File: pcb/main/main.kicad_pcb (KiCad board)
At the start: 2 copper layers, 29.4 x 98.3 mm, 54 parts, among them J1 Conn_01x04, J2 USB_B, J3 Serial, J4 STLink, J5 RJ45, J6 SELECT, J7 READ, J8 TRACKBALL, SW5 RST_SW, SW6 BOOT0, SW7 BOOT1, U1 3.3v regul, U2 STM32F103C8Tx, Y1 32.768kHz, Y2 8MHz

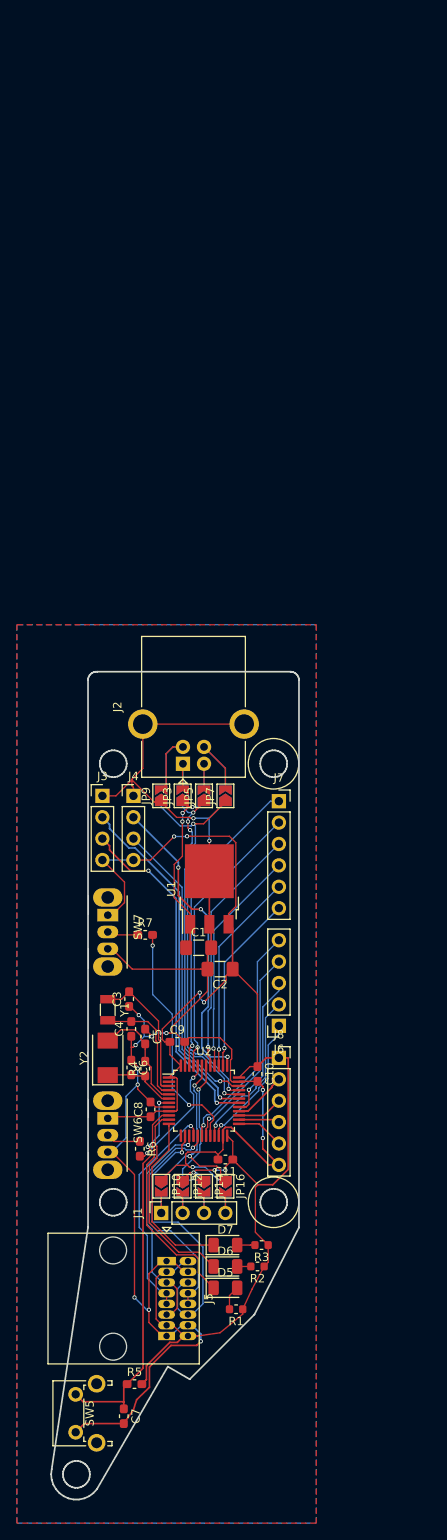
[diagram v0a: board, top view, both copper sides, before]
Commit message: fix pcb
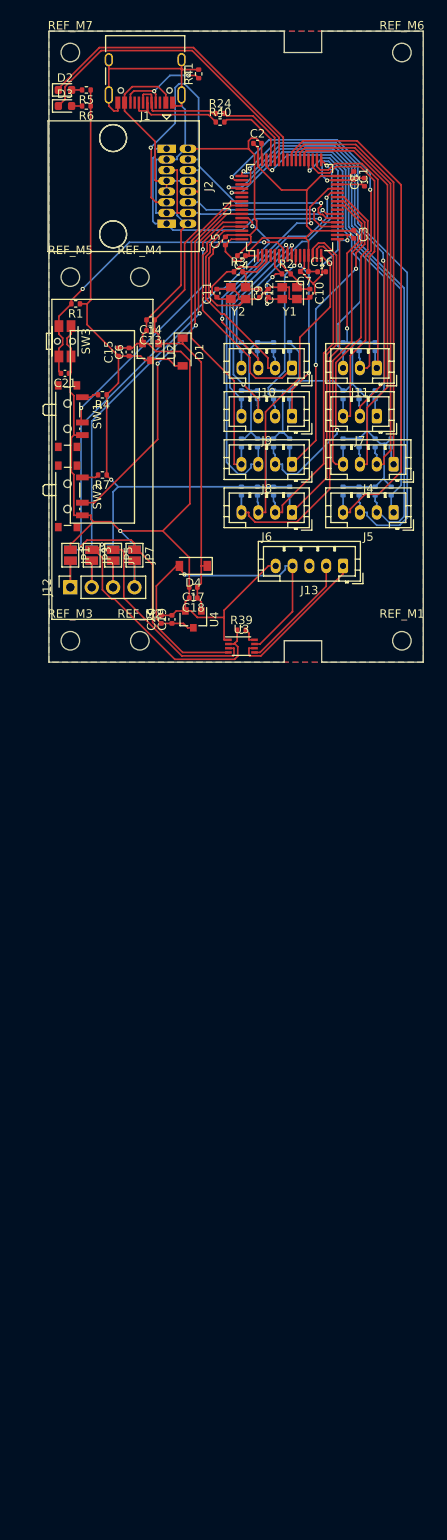
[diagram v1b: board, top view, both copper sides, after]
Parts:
- removed D5, D6, D7: LED, LED_SMD:LED_1206_3216Metric
- removed G*** (x2): LOGO, folivora:logo
- removed JP10, JP12, JP14, JP16, JP9: R, Jumper:SolderJumper-2_P1.3mm_Open_TrianglePad1.0x1.5mm
- removed JP11, JP13, JP15, JP17: L, Jumper:SolderJumper-2_P1.3mm_Open_TrianglePad1.0x1.5mm
- removed SW5: RST_SW, Button_Switch_THT:SW_Tactile_SPST_Angled_PTS645Vx31-2LFS
- removed SW6: BOOT0, Button_Switch_THT:SW_CuK_OS102011MA1QN1_SPDT_Angled
- removed SW7: BOOT1, Button_Switch_THT:SW_CuK_OS102011MA1QN1_SPDT_Angled
- added C12: C, Capacitor_SMD:C_0402_1005Metric, F.Cu at (25.0, -43.8)
- added C13: 1uF, Capacitor_SMD:C_0402_1005Metric, F.Cu at (12.1, -39.4)
- added C14: 0.1uF, Capacitor_SMD:C_0402_1005Metric, F.Cu at (12.1, -40.6)
- added C15: 0.1uF, Capacitor_SMD:C_0402_1005Metric, F.Cu at (8.26, -36.8)
- added C16: 1uF, Capacitor_SMD:C_0402_1005Metric, F.Cu at (32.4, -46.4)
- added C17: 1uF, Capacitor_SMD:C_0402_1005Metric, F.Cu at (17.1, -8.89)
- added C18: 0.1uF, Capacitor_SMD:C_0402_1005Metric, F.Cu at (17.1, -7.62)
- added C19: 0.1uF, Capacitor_SMD:C_0402_1005Metric, F.Cu at (14.6, -5.08)
- added C20: 1uF, Capacitor_SMD:C_0402_1005Metric, F.Cu at (13.3, -5.08)
- added C21: 0.1uF, Capacitor_SMD:C_0402_1005Metric, F.Cu at (1.91, -34.3)
- added D1: SBD, Diode_SMD:D_SOD-123, F.Cu at (15.9, -36.8)
- added D2: Error, LED_SMD:LED_0603_1608Metric, F.Cu at (1.91, -67.9)
- added D3: Status, LED_SMD:LED_0603_1608Metric, F.Cu at (1.91, -66.0)
- added D4: SBD, Diode_SMD:D_SOD-123, F.Cu at (17.1, -11.4)
- added J10: COL4, Connector_JST:JST_PH_B4B-PH-K_1x04_P2.00mm_Vertical, F.Cu at (28.9, -34.9)
- added J11: COL6, Connector_JST:JST_PH_B3B-PH-K_1x03_P2.00mm_Vertical, F.Cu at (38.9, -34.9)
- added J12: OLED, folivora:OLED, F.Cu at (6.35, -8.89)
- added J13: Conn_01x05_Female, Connector_JST:JST_PH_B5B-PH-K_1x05_P2.00mm_Vertical, F.Cu at (34.9, -11.4)
- added J9: COL3, Connector_JST:JST_PH_B4B-PH-K_1x04_P2.00mm_Vertical, F.Cu at (28.9, -29.2)
- added JP1: OLED_1_F, Jumper:SolderJumper-2_P1.3mm_Open_Pad1.0x1.5mm, F.Cu at (2.54, -12.7)
- added R10: 10k, Resistor_SMD:R_0402_1005Metric, B.Cu at (36.8, -20.3)
- added R11: 10k, Resistor_SMD:R_0402_1005Metric, B.Cu at (34.9, -20.3)
- added R12: 10k, Resistor_SMD:R_0402_1005Metric, B.Cu at (40.6, -26.0)
- added R13: 10k, Resistor_SMD:R_0402_1005Metric, B.Cu at (38.7, -26.0)
- added R14: 10k, Resistor_SMD:R_0402_1005Metric, B.Cu at (36.8, -26.0)
- added R15: 10k, Resistor_SMD:R_0402_1005Metric, B.Cu at (34.9, -26.0)
- added R16: 10k, Resistor_SMD:R_0402_1005Metric, B.Cu at (28.6, -31.8)
- added R17: 10k, Resistor_SMD:R_0402_1005Metric, B.Cu at (26.7, -31.8)
- added R18: 10k, Resistor_SMD:R_0402_1005Metric, B.Cu at (24.8, -31.8)
- added R19: 10k, Resistor_SMD:R_0402_1005Metric, B.Cu at (22.9, -31.8)
- added R20: 10k, Resistor_SMD:R_0402_1005Metric, B.Cu at (34.9, -37.5)
- added R21: 10k, Resistor_SMD:R_0402_1005Metric, B.Cu at (36.8, -37.5)
- added R22: 10k, Resistor_SMD:R_0402_1005Metric, B.Cu at (38.7, -37.5)
- added R23: 10k, Resistor_SMD:R_0402_1005Metric, B.Cu at (22.9, -37.5)
- added R24: 10, Resistor_SMD:R_0402_1005Metric, F.Cu at (20.3, -65.2)
- added R25: 10k, Resistor_SMD:R_0402_1005Metric, B.Cu at (24.8, -37.5)
- added R26: 10k, Resistor_SMD:R_0402_1005Metric, B.Cu at (26.7, -37.5)
- added R27: 10k, Resistor_SMD:R_0402_1005Metric, B.Cu at (28.6, -37.5)
- added R28: 10k, Resistor_SMD:R_0402_1005Metric, B.Cu at (22.9, -26.0)
- added R29: 10k, Resistor_SMD:R_0402_1005Metric, B.Cu at (24.8, -26.0)
- added R30: 10k, Resistor_SMD:R_0402_1005Metric, B.Cu at (26.7, -26.0)
- added R31: 10k, Resistor_SMD:R_0402_1005Metric, B.Cu at (28.6, -26.0)
- added R32: 10k, Resistor_SMD:R_0402_1005Metric, B.Cu at (34.9, -31.8)
- added R33: 10k, Resistor_SMD:R_0402_1005Metric, B.Cu at (36.8, -31.8)
- added R34: 10k, Resistor_SMD:R_0402_1005Metric, B.Cu at (38.7, -31.8)
- added R35: 10k, Resistor_SMD:R_0402_1005Metric, B.Cu at (22.9, -20.3)
- added R36: 10k, Resistor_SMD:R_0402_1005Metric, B.Cu at (24.8, -20.3)
- added R37: 10k, Resistor_SMD:R_0402_1005Metric, B.Cu at (26.7, -20.3)
- added R38: 10k, Resistor_SMD:R_0402_1005Metric, B.Cu at (28.6, -20.3)
- added R39: R, Resistor_SMD:R_0402_1005Metric, F.Cu at (22.9, -3.81)
- added R40: 10, Resistor_SMD:R_0402_1005Metric, F.Cu at (20.3, -64.1)
- added R41: 5.1k, Resistor_SMD:R_0402_1005Metric, F.Cu at (17.8, -69.8)
- added R8: 10k, Resistor_SMD:R_0402_1005Metric, B.Cu at (40.6, -20.3)
- added R9: 10k, Resistor_SMD:R_0402_1005Metric, B.Cu at (38.7, -20.3)
- added REF_M1: MountingHole_2.2mm_M2, MountingHole:MountingHole_2.2mm_M2, F.Cu at (41.9, -2.54)
- added REF_M2: MountingHole_2.2mm_M2, MountingHole:MountingHole_2.2mm_M2, F.Cu at (10.8, -2.54)
- added REF_M3: MountingHole_2.2mm_M2, MountingHole:MountingHole_2.2mm_M2, F.Cu at (2.54, -2.54)
- added REF_M4: MountingHole_2.2mm_M2, MountingHole:MountingHole_2.2mm_M2, F.Cu at (10.8, -45.7)
- added REF_M5: MountingHole_2.2mm_M2, MountingHole:MountingHole_2.2mm_M2, F.Cu at (2.54, -45.7)
- added REF_M6: MountingHole_2.2mm_M2, MountingHole:MountingHole_2.2mm_M2, F.Cu at (41.9, -72.4)
- added REF_M7: MountingHole_2.2mm_M2, MountingHole:MountingHole_2.2mm_M2, F.Cu at (2.54, -72.4)
- added SW1: SW_SPDT, Button_Switch_SMD:SW_SPDT_PCM12, F.Cu at (2.54, -29.2)
- added SW2: SW_SPDT, Button_Switch_SMD:SW_SPDT_PCM12, F.Cu at (2.54, -19.7)
- added SW3: RESET, Button_Switch_SMD:SW_SPST_EVQP7C, F.Cu at (1.91, -38.1)
- added U3: PCA9306DC1, Package_SO:VSSOP-8_2.3x2mm_P0.5mm, F.Cu at (22.9, -1.91)
- added U4: HT7727, Package_TO_SOT_SMD:SOT-23, F.Cu at (17.1, -5.08)
- C1, C2: value 10uF -> 0.1uF; footprint Capacitor_SMD:C_1206_3216Metric_Pad1.42x1.75mm_HandSolder -> Capacitor_SMD:C_0402_1005Metric
- C10, C11, C9: value 0.1uF -> C; footprint Capacitor_SMD:C_0603_1608Metric_Pad1.05x0.95mm_HandSolder -> Capacitor_SMD:C_0402_1005Metric
- C3: value 12.5pF -> 0.1uF; footprint Capacitor_SMD:C_0603_1608Metric_Pad1.05x0.95mm_HandSolder -> Capacitor_SMD:C_0402_1005Metric
- C4: value 12.5pF[ -> 0.1uF; footprint Capacitor_SMD:C_0603_1608Metric_Pad1.05x0.95mm_HandSolder -> Capacitor_SMD:C_0402_1005Metric
- C5: value 20pF -> 0.1uF; footprint Capacitor_SMD:C_0603_1608Metric_Pad1.05x0.95mm_HandSolder -> Capacitor_SMD:C_0402_1005Metric
- C6: value 20pF -> 1uF; footprint Capacitor_SMD:C_0603_1608Metric_Pad1.05x0.95mm_HandSolder -> Capacitor_SMD:C_0402_1005Metric
- C7: value 10uF -> 10nF; footprint Capacitor_SMD:C_0603_1608Metric_Pad1.05x0.95mm_HandSolder -> Capacitor_SMD:C_0402_1005Metric
- C8: value 0.1uF -> 4.7uF; footprint Capacitor_SMD:C_0603_1608Metric_Pad1.05x0.95mm_HandSolder -> Capacitor_SMD:C_0402_1005Metric
- J1: value Conn_01x04 -> USB_C_Receptacle_USB2.0; footprint Connector_PinSocket_2.54mm:PinSocket_1x04_P2.54mm_Vertical -> Connector_USB:USB_C_Receptacle_HRO_TYPE-C-31-M-12
- J2: value USB_B -> RJ45; footprint Connector_USB:USB_B_OST_USB-B1HSxx_Horizontal -> folivora:RJ45_rev
- J3: value Serial -> RJ45; footprint Connector_PinHeader_2.54mm:PinHeader_1x04_P2.54mm_Vertical -> folivora:RJ45_rev; moved to B.Cu
- J4: value STLink -> Pad; footprint Connector_PinHeader_2.54mm:PinHeader_1x04_P2.54mm_Vertical -> Connector_JST:JST_PH_B4B-PH-K_1x04_P2.00mm_Vertical
- J5: value RJ45 -> Thumb; footprint folivora:RJ45_rev -> Connector_JST:JST_PH_B4B-PH-K_1x04_P2.00mm_Vertical
- J6: value SELECT -> COL1; footprint Connector_PinSocket_2.54mm:PinSocket_1x05_P2.54mm_Vertical -> Connector_JST:JST_PH_B4B-PH-K_1x04_P2.00mm_Vertical
- J7: value READ -> COL5; footprint Connector_PinSocket_2.54mm:PinSocket_1x06_P2.54mm_Vertical -> Connector_JST:JST_PH_B3B-PH-K_1x03_P2.00mm_Vertical
- J8: value TRACKBALL -> COL2; footprint Connector_PinSocket_2.54mm:PinSocket_1x06_P2.54mm_Vertical -> Connector_JST:JST_PH_B4B-PH-K_1x04_P2.00mm_Vertical
- JP2: value L -> OLED_1_B; footprint Jumper:SolderJumper-2_P1.3mm_Open_TrianglePad1.0x1.5mm -> Jumper:SolderJumper-2_P1.3mm_Open_Pad1.0x1.5mm
- JP3: value R -> OLED_2_F; footprint Jumper:SolderJumper-2_P1.3mm_Open_TrianglePad1.0x1.5mm -> Jumper:SolderJumper-2_P1.3mm_Open_Pad1.0x1.5mm
- JP4: value L -> OLED_2_B; footprint Jumper:SolderJumper-2_P1.3mm_Open_TrianglePad1.0x1.5mm -> Jumper:SolderJumper-2_P1.3mm_Open_Pad1.0x1.5mm
- JP5: value R -> OLED_3_F; footprint Jumper:SolderJumper-2_P1.3mm_Open_TrianglePad1.0x1.5mm -> Jumper:SolderJumper-2_P1.3mm_Open_Pad1.0x1.5mm
- JP6: value L -> OLED_3_B; footprint Jumper:SolderJumper-2_P1.3mm_Open_TrianglePad1.0x1.5mm -> Jumper:SolderJumper-2_P1.3mm_Open_Pad1.0x1.5mm
- JP7: value R -> OLED_4_F; footprint Jumper:SolderJumper-2_P1.3mm_Open_TrianglePad1.0x1.5mm -> Jumper:SolderJumper-2_P1.3mm_Open_Pad1.0x1.5mm
- JP8: value L -> OLED_4_B; footprint Jumper:SolderJumper-2_P1.3mm_Open_TrianglePad1.0x1.5mm -> Jumper:SolderJumper-2_P1.3mm_Open_Pad1.0x1.5mm
- R1: footprint Resistor_SMD:R_0603_1608Metric -> Resistor_SMD:R_0402_1005Metric
- R2, R3: value R -> 10M; footprint Resistor_SMD:R_0603_1608Metric -> Resistor_SMD:R_0402_1005Metric
- R4: value 10Mohm -> R; footprint Resistor_SMD:R_0603_1608Metric_Pad1.05x0.95mm_HandSolder -> Resistor_SMD:R_0402_1005Metric
- R5, R6, R7: value 10kohm -> R; footprint Resistor_SMD:R_0603_1608Metric_Pad1.05x0.95mm_HandSolder -> Resistor_SMD:R_0402_1005Metric
- U1: value 3.3v regul -> STM32F401RETx; footprint Package_TO_SOT_SMD:TO-252-3_TabPin2 -> Package_QFP:LQFP-64_10x10mm_P0.5mm
- U2: value STM32F103C8Tx -> NATLINEAR XT1861B332MR-G; footprint Package_QFP:LQFP-48_7x7mm_P0.5mm -> Package_TO_SOT_SMD:SOT-23
- Y1: value 32.768kHz -> Crystal_8MHz; footprint Crystal:Crystal_SMD_3215-2Pin_3.2x1.5mm -> Crystal:Crystal_SMD_2520-4Pin_2.5x2.0mm
- Y2: value 8MHz -> Crystal_32.768MHz; footprint Crystal:Crystal_SMD_Abracon_ABM3-2Pin_5.0x3.2mm -> Crystal:Crystal_SMD_2520-4Pin_2.5x2.0mm
- moved R5 153.8 mm to (4.45, -67.9), turned to 180 degrees
- moved C7 137.6 mm to (30.3, -46.4), turned to 180 degrees
- moved J1 135.9 mm to (11.4, -70.5), turned to 180 degrees
- moved R6 124.0 mm to (4.45, -66.0), turned to 180 degrees
- moved R1 120.9 mm to (3.17, -42.5)
- moved R2 117.9 mm to (28.2, -46.1), turned to 0 degrees
- moved R3 115.6 mm to (22.5, -46.4), turned to 0 degrees
- moved C8 113.0 mm to (37.5, -57.0)
- moved C11 102.9 mm to (19.9, -43.8), turned to 90 degrees
- moved C2 98.1 mm to (24.8, -61.6), turned to 0 degrees
- moved C5 94.9 mm to (21.0, -50.0), turned to 90 degrees
- moved C3 94.6 mm to (36.2, -50.8), turned to 270 degrees
- moved C1 93.5 mm to (36.2, -57.8), turned to 270 degrees
- moved C10 92.9 mm to (31.0, -43.8)
- moved J5 92.9 mm to (40.9, -17.8), turned to 180 degrees
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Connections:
- C1 pad 1: +5V -> +3V3
- C10 pad 1: +3V3 -> /XTAL1B
- C11 pad 1: +3V3 -> /XTAL2A
- C3 pad 1: GND -> +3V3
- C3 pad 2: /XTAL_C -> GND
- C4 pad 1: GND -> +3V3
- C4 pad 2: /XTAL_D -> GND
- C5 pad 1: GND -> +3V3
- C5 pad 2: /XTAL_A -> GND
- C6 pad 1: GND -> +3V3
- C6 pad 2: /XTAL_B -> GND
- C7 pad 1: /RST -> +3V3
- C8 pad 1: +3V3 -> Net-(C8-Pad1)
- C9 pad 1: +3V3 -> /XTAL1A
- J2 pad 1: /USB_1 -> /SCLK
- J2 pad 2: /USB_2 -> /MISO
- J2 pad 3: /USB_3 -> /MOSI
- J2 pad 4: /USB_4 -> VBUS
- J2 pad 5: GND -> VBUS
- J3 pad 1: GND -> /SCLK
- J3 pad 2: /RX -> /MOSI
- J3 pad 3: /TX -> /MISO
- J3 pad 4: +3V3 -> VBUS
- J4 pad 1: GND -> Net-(J4-Pad1)
- J4 pad 2: /SWCLK -> Net-(J4-Pad2)
- J4 pad 3: /SWDIO -> Net-(J4-Pad3)
- J4 pad 4: +3V3 -> Net-(J4-Pad4)
- J5 pad 1: GND -> Net-(J5-Pad1)
- J5 pad 2: GND -> Net-(J5-Pad2)
- J5 pad 3: /SCK -> Net-(J5-Pad3)
- J5 pad 4: /MOSI -> Net-(J5-Pad4)
- J6 pad 1: /SELECT0 -> Net-(J6-Pad1)
- J6 pad 2: /SELECT1 -> Net-(J6-Pad2)
- J6 pad 3: /SELECT2 -> Net-(J6-Pad3)
- J6 pad 4: /SELECT3 -> Net-(J6-Pad4)
- J7 pad 1: /READ0 -> Net-(J7-Pad1)
- J7 pad 2: /READ1 -> Net-(J7-Pad2)
- J7 pad 3: /READ2 -> Net-(J7-Pad3)
- J8 pad 1: +3V3 -> Net-(J8-Pad1)
- J8 pad 2: /UP -> Net-(J8-Pad2)
- J8 pad 3: /DOWN -> Net-(J8-Pad3)
- J8 pad 4: /RIGHT -> Net-(J8-Pad4)
- JP2 pad 1: /D- -> /SDA
- JP2 pad 2: /USB_1 -> /OLED1
- JP3 pad 1: +5V -> +3V3
- JP3 pad 2: /USB_1 -> /OLED2
- JP4 pad 1: +5V -> /SCL
- JP4 pad 2: /USB_2 -> /OLED2
- JP5 pad 1: /D- -> /SCL
- JP5 pad 2: /USB_2 -> /OLED3
- JP6 pad 1: GND -> +3V3
- JP6 pad 2: /USB_3 -> /OLED3
- JP7 pad 1: /D+ -> /SDA
- JP7 pad 2: /USB_3 -> /OLED4
- JP8 pad 1: /D+ -> GND
- JP8 pad 2: /USB_4 -> /OLED4
- R1 pad 2: Net-(D5-Pad2) -> Net-(C21-Pad2)
- R2 pad 1: +3V3 -> /XTAL1A
- R2 pad 2: Net-(D6-Pad2) -> /XTAL1B
- R3 pad 1: +3V3 -> /XTAL2A
- R3 pad 2: Net-(D7-Pad2) -> /XTAL2B
- R4 pad 1: /XTAL_B -> +3V3
- R4 pad 2: /XTAL_A -> Net-(R4-Pad2)
- R5 pad 1: /RST -> +3V3
- R5 pad 2: +3V3 -> Net-(D2-Pad2)
- R6 pad 1: Net-(R6-Pad1) -> +3V3
- R6 pad 2: /BOOT0 -> Net-(D3-Pad2)
- R7 pad 1: Net-(R7-Pad1) -> +3V3
- R7 pad 2: /BOOT1 -> Net-(R7-Pad2)
- U1 pad 1: +5V -> +3V3
- U1 pad 2: GND -> /XTAL2A
- U1 pad 3: +3V3 -> /XTAL2B
- U2 pad 1: +3V3 -> VBUS
- U2 pad 2: Net-(U2-Pad2) -> GND
- U2 pad 3: /XTAL_C -> +3V3
- Y1 pad 1: /XTAL_D -> /XTAL1B
- Y1 pad 2: /XTAL_C -> GND
- Y2 pad 1: /XTAL_B -> /XTAL2B
- Y2 pad 2: /XTAL_A -> GND
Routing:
- net +3V3: track 175.5 -> 265.0 mm, vias 7 -> 3
- net VBUS: track 0.00 -> 85.0 mm
- net Net-(J5-Pad3): track 0.00 -> 71.3 mm, vias 0 -> 1
- net Net-(J5-Pad2): track 0.00 -> 69.3 mm, vias 0 -> 1
- net Net-(J5-Pad1): track 0.00 -> 61.9 mm, vias 0 -> 1
- net Net-(J5-Pad4): track 0.00 -> 61.8 mm
- net /SDA: track 22.1 -> 80.4 mm
- net /SCL: track 17.7 -> 75.3 mm
- net Net-(J7-Pad3): track 0.00 -> 54.1 mm, vias 0 -> 2
- net Net-(J7-Pad2): track 0.00 -> 50.7 mm, vias 0 -> 2
- net Net-(J4-Pad1): track 0.00 -> 50.4 mm
- net Net-(J4-Pad2): track 0.00 -> 50.2 mm
- net Net-(J4-Pad3): track 0.00 -> 49.6 mm
- net Net-(J8-Pad3): track 0.00 -> 46.5 mm, vias 0 -> 1
- net /RST: track 45.7 -> 0.00 mm, vias 2 -> 0
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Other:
- board size 29.4 x 98.3 mm -> 44.5 x 74.9 mm
